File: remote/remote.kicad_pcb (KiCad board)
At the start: 2 copper layers, 42 x 28 mm, 6 parts, among them J1 Conn_01x10_Pin, SW1 SW_Push, SW2 SW_Push, U1 STM32L051C8Tx

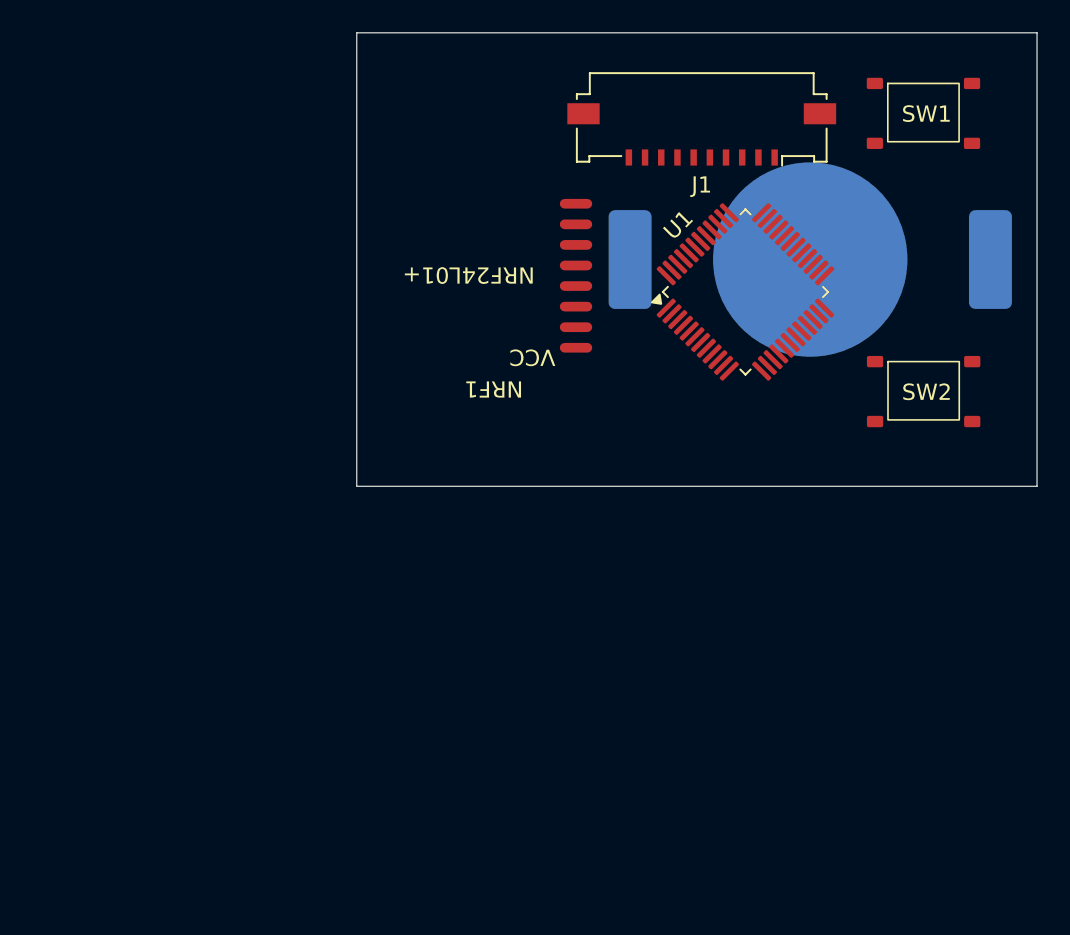
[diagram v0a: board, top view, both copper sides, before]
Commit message: New versions
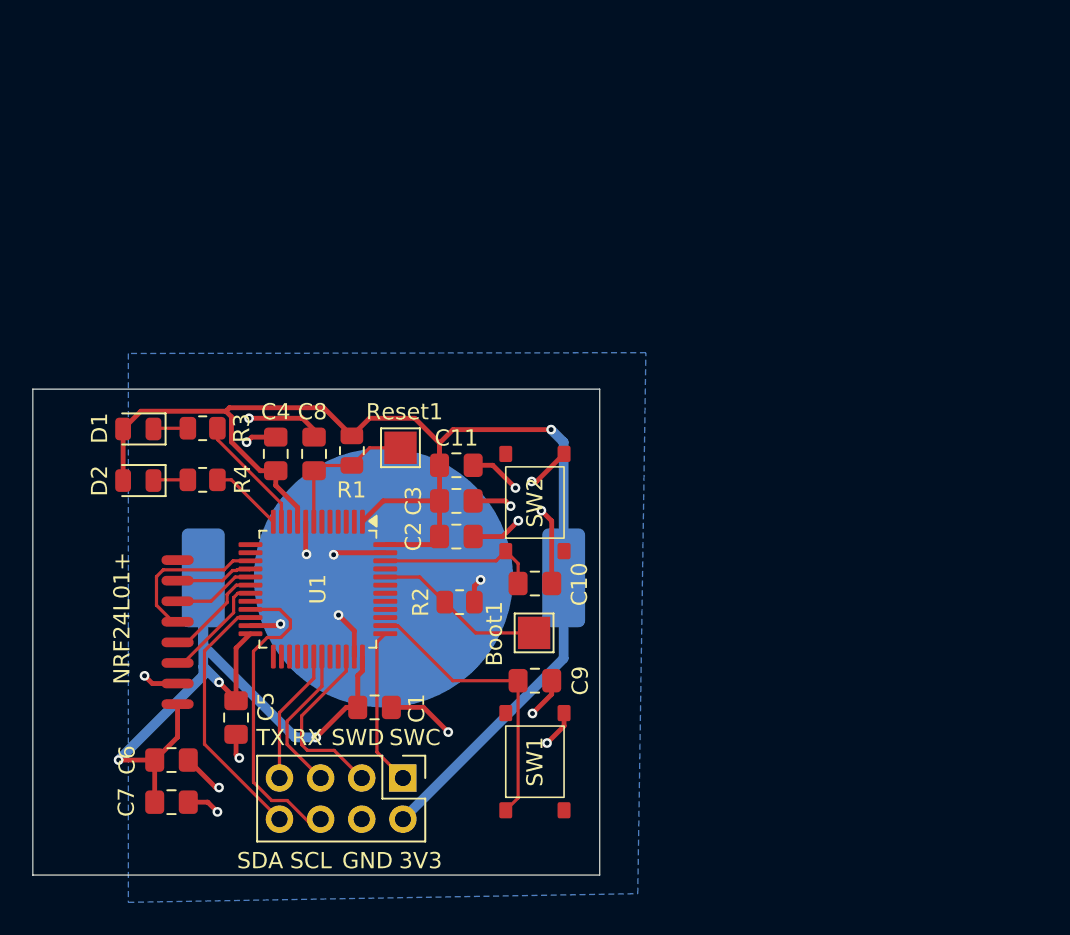
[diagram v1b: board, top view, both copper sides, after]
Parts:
- added Boot1: TestPoint, TestPoint:TestPoint_Pad_2.0x2.0mm, F.Cu at (130.9, 115.0)
- added C1: 100n, Capacitor_SMD:C_0805_2012Metric_Pad1.18x1.45mm_HandSolder, F.Cu at (121.1, 119.7)
- added C10: 100n, Capacitor_SMD:C_0805_2012Metric_Pad1.18x1.45mm_HandSolder, F.Cu at (131.0, 112.0)
- added C11: 4.7u, Capacitor_SMD:C_0805_2012Metric_Pad1.18x1.45mm_HandSolder, F.Cu at (126.2, 104.7)
- added C2: 100n, Capacitor_SMD:C_0805_2012Metric_Pad1.18x1.45mm_HandSolder, F.Cu at (126.2, 109.1)
- added C3: 100n, Capacitor_SMD:C_0805_2012Metric_Pad1.18x1.45mm_HandSolder, F.Cu at (126.2, 106.9)
- added C4: 100n, Capacitor_SMD:C_0805_2012Metric_Pad1.18x1.45mm_HandSolder, F.Cu at (115.0, 104.0)
- added C5: 100n, Capacitor_SMD:C_0805_2012Metric_Pad1.18x1.45mm_HandSolder, F.Cu at (112.5, 120.3)
- added C6: 4.7u, Capacitor_SMD:C_0805_2012Metric_Pad1.18x1.45mm_HandSolder, F.Cu at (108.6, 122.9)
- added C7: 100n, Capacitor_SMD:C_0805_2012Metric_Pad1.18x1.45mm_HandSolder, F.Cu at (108.6, 125.5)
- added C8: 100n, Capacitor_SMD:C_0805_2012Metric_Pad1.18x1.45mm_HandSolder, F.Cu at (117.4, 104.0)
- added C9: 100n, Capacitor_SMD:C_0805_2012Metric_Pad1.18x1.45mm_HandSolder, F.Cu at (131.0, 118.0)
- added D1: LED, LED_SMD:LED_0805_2012Metric, F.Cu at (106.5, 102.5)
- added D2: LED, LED_SMD:LED_0805_2012Metric, F.Cu at (106.5, 105.6)
- added R1: 100k, Resistor_SMD:R_0805_2012Metric, F.Cu at (119.7, 103.8)
- added R2: 100k, Resistor_SMD:R_0805_2012Metric, F.Cu at (126.3, 113.2)
- added R3: 10k, Resistor_SMD:R_0805_2012Metric, F.Cu at (110.5, 102.4)
- added R4: 10k, Resistor_SMD:R_0805_2012Metric, F.Cu at (110.5, 105.6)
- added Reset1: TestPoint, TestPoint:TestPoint_Pad_2.0x2.0mm, F.Cu at (122.7, 103.6)
- J1: value Conn_01x10_Pin -> Conn_01x08_Pin; footprint Connector_FFC-FPC:Molex_200528-0100_1x10-1MP_P1.00mm_Horizontal -> Connector_PinHeader_2.54mm:PinHeader_2x04_P2.54mm_Vertical
- moved J1 43.3 mm to (122.8, 124.0), turned to -90 degrees
- moved SW2 33.3 mm to (131.0, 107.0), turned to 90 degrees
- moved NRF1 33.0 mm to (108.9, 119.4)
- moved BT1 32.9 mm to (121.7, 111.7)
- moved SW1 32.4 mm to (131.0, 123.0), turned to 90 degrees
- moved U1 32.2 mm to (117.6, 112.3), turned to -90 degrees
- renumbered SW2 to SW1, SW1 to SW2
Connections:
- BT1 pad 1: unconnected-(BT1-+-Pad1) -> +3V3
- BT1 pad 2: unconnected-(BT1---Pad2) -> GND
- J1 pad 1: /GND -> /SWCLK
- J1 pad 2: /3V3 -> +3V3
- J1 pad 3: /SWCLK -> /SWDIO
- J1 pad 4: /SWDIO -> GND
- J1 pad 5: /UART_RX -> /USART1_RX
- J1 pad 6: /UART_TX -> /SCL
- J1 pad 7: /Boot -> /USART1_TX
- J1 pad 8: /Reset -> /SDA
- NRF1 pad 1: unconnected-(NRF1-VCC-Pad1) -> +3V3
- NRF1 pad 2: unconnected-(NRF1-GND-Pad2) -> GND
- NRF1 pad 3: unconnected-(NRF1-CE-Pad3) -> /SPI_CE
- NRF1 pad 4: unconnected-(NRF1-CSN-Pad4) -> /SPI_CSN
- NRF1 pad 5: unconnected-(NRF1-SCK-Pad5) -> /SPI_SCK
- NRF1 pad 6: unconnected-(NRF1-MOSI-Pad6) -> /SPI_MOSI
- NRF1 pad 7: unconnected-(NRF1-MISO-Pad7) -> /SPI_MISO
- SW1 pad 1: unconnected-(SW2-Pad1) -> /SW1
- SW1 pad 2: unconnected-(SW2-Pad2) -> GND
- SW2 pad 1: unconnected-(SW1-Pad1) -> /SW2
- SW2 pad 2: unconnected-(SW1-Pad2) -> GND
- U1 pad 1: unconnected-(U1-VDD-Pad1) -> +3V3
- U1 pad 10: unconnected-(U1-PA0-Pad10) -> /ADC_V_EXT
- U1 pad 11: unconnected-(U1-PA1-Pad11) -> /LED_RED
- U1 pad 12: unconnected-(U1-PA2-Pad12) -> /LED_GREEN
- U1 pad 15: unconnected-(U1-PA5-Pad15) -> /SPI_SCK
- U1 pad 16: unconnected-(U1-PA6-Pad16) -> /SPI_MISO
- U1 pad 17: unconnected-(U1-PA7-Pad17) -> /SPI_MOSI
- U1 pad 18: unconnected-(U1-PB0-Pad18) -> /SPI_CSN
- U1 pad 19: unconnected-(U1-PB1-Pad19) -> /SPI_CE
- U1 pad 21: unconnected-(U1-PB10-Pad21) -> /SCL
- U1 pad 22: unconnected-(U1-PB11-Pad22) -> /SDA
- U1 pad 23: Net-(U1-VSS-Pad23) -> GND
- U1 pad 24: unconnected-(U1-VDD-Pad24) -> +3V3
- U1 pad 30: unconnected-(U1-PA9-Pad30) -> /USART1_TX
- U1 pad 31: unconnected-(U1-PA10-Pad31) -> /USART1_RX
- U1 pad 34: unconnected-(U1-PA13-Pad34) -> /SWDIO
- U1 pad 35: Net-(U1-VSS-Pad23) -> GND
- U1 pad 36: unconnected-(U1-VDDIO2-Pad36) -> +3V3
- U1 pad 37: unconnected-(U1-PA14-Pad37) -> /SWCLK
- U1 pad 38: unconnected-(U1-PA15-Pad38) -> /SW1
- U1 pad 44: unconnected-(U1-BOOT0-Pad44) -> /BOOT
- U1 pad 46: unconnected-(U1-PB9-Pad46) -> /SW2
- U1 pad 47: Net-(U1-VSS-Pad23) -> GND
- U1 pad 48: unconnected-(U1-VDD-Pad48) -> +3V3
- U1 pad 7: unconnected-(U1-NRST-Pad7) -> /RESET
- U1 pad 8: unconnected-(U1-VSSA-Pad8) -> GND
- U1 pad 9: unconnected-(U1-VDDA-Pad9) -> +3V3
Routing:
- net +3V3: track 0.00 -> 141.5 mm, vias 0 -> 4
- net GND: track 0.00 -> 53.0 mm, vias 0 -> 19
- net /SCL: track 0.00 -> 18.8 mm
- net /SW1: track 0.00 -> 17.9 mm
- net /SDA: track 0.00 -> 16.0 mm
- net /SWDIO: track 0.00 -> 11.1 mm
- net /BOOT: track 0.00 -> 10.6 mm
- net /SW2: track 0.00 -> 10.0 mm
- net /SWCLK: track 0.00 -> 9.79 mm
- net /SPI_SCK: track 0.00 -> 9.70 mm
- net /USART1_RX: track 0.00 -> 9.36 mm
- net /RESET: track 0.00 -> 9.08 mm
- net /USART1_TX: track 0.00 -> 8.47 mm
- net /LED_RED: track 0.00 -> 7.41 mm
- net /SPI_CE: track 0.00 -> 6.83 mm
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- added copper zone on B.Cu, net GND
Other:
- board size 42 x 28 mm -> 35 x 30 mm
- board text added: "3V3"
- board text added: "GND"
- board text added: "RX"
- board text added: "SCL"
- board text added: "SDA"
- board text added: "SWC"
- board text added: "SWD"
- board text added: "TX"
